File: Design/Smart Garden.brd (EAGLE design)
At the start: 92 x 87 mm, 96 parts, among them IC2 MP1584EN-LF-Z, IC3 CP2102, J1 USB-C, J2 POWER_JACK, T1 MMBT3904, T2 MMBT3904, T3 MMBT2222A, T4 MMBT2222A, T5 MMBT2222A, T6 MMBT2222A, U1 ESP-32S, U3 LM2596S, U4 DB107S

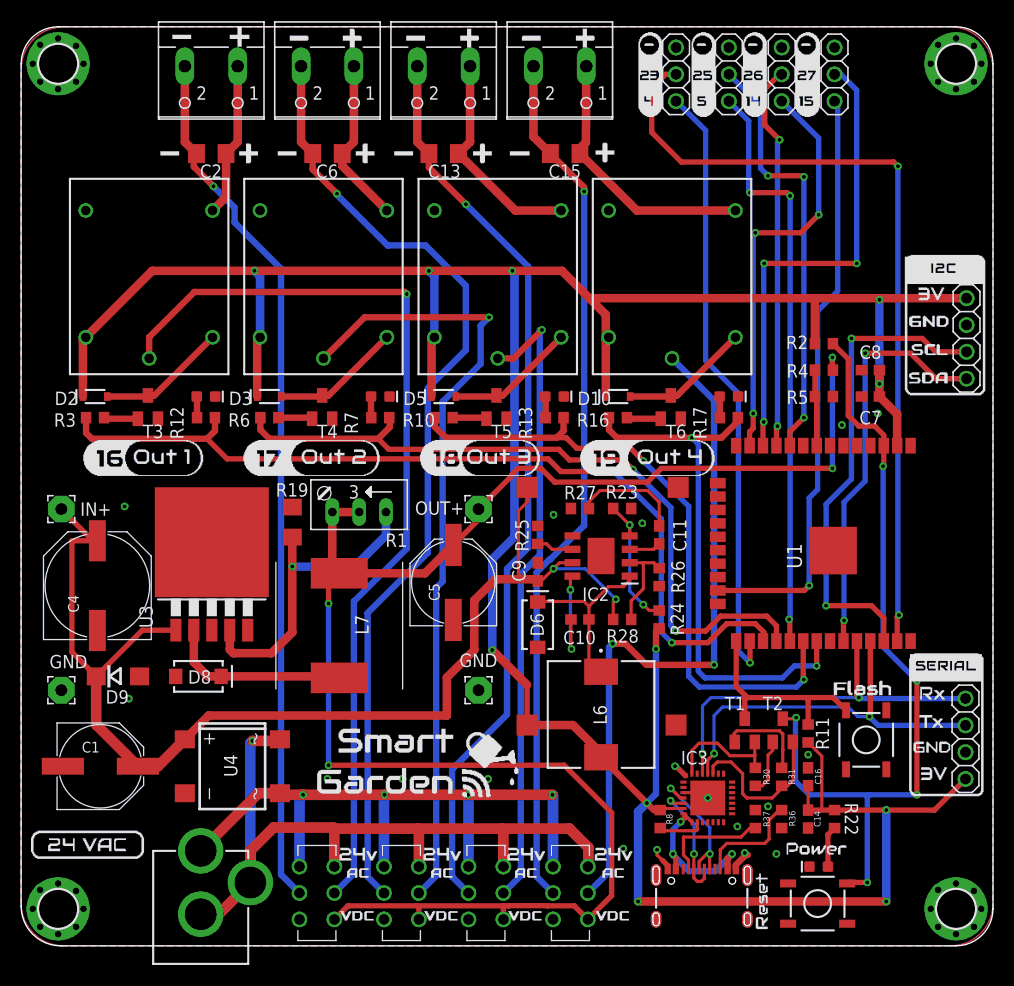
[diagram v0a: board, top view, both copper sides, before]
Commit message: Added V2R1 design files
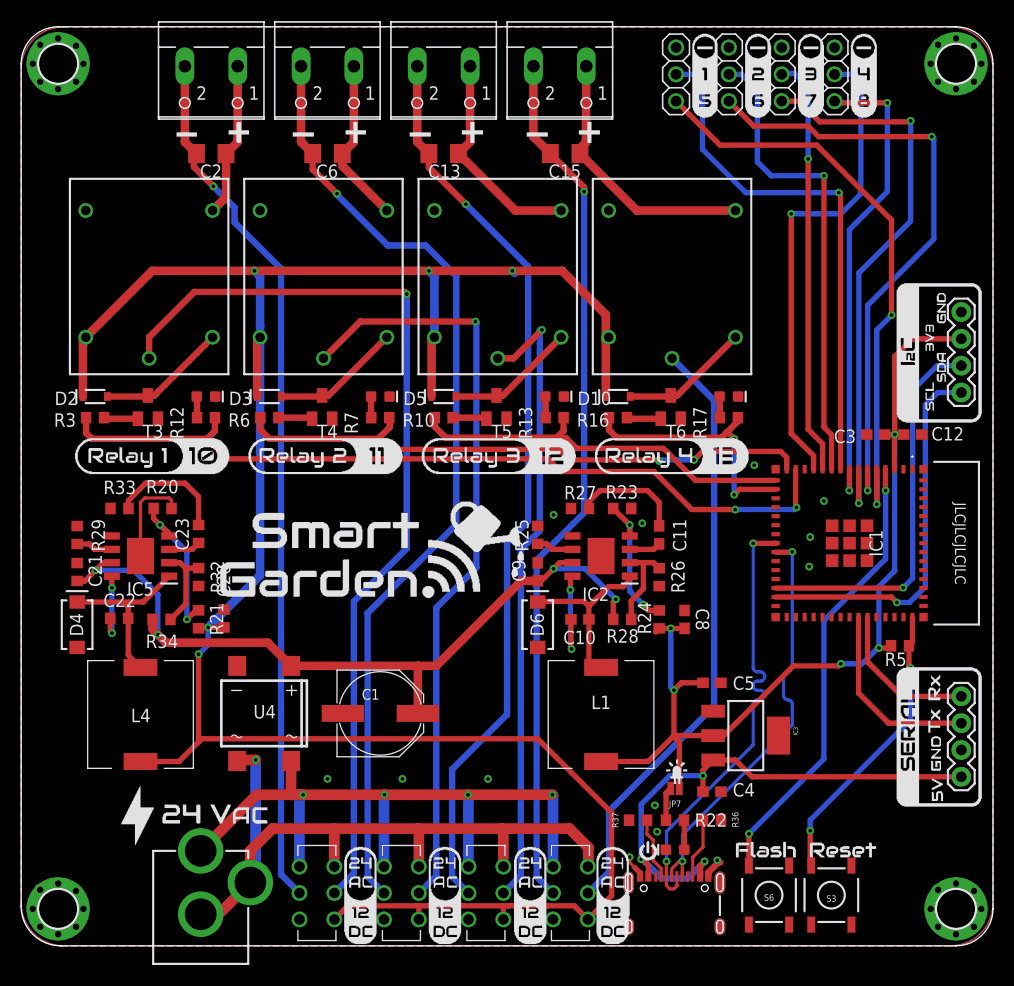
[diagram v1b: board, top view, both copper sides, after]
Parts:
- removed C14: 0.1uF, rcl:C0603
- removed C16: 4.7uF, rcl:C0603
- removed C7: 100nF, rcl:C0603
- removed D8: 3A/40V/500mV, SparkFun-DiscreteSemi:SMA-DIODE
- removed D9: US1M, diode:DO214AC
- removed JP1: Serial, SpaceDIY_connectors:1X04
- removed JP6: I2C, SpaceDIY_connectors:1X04
- removed L6: SLF10145T-100M2R5-H, SamacSys_Parts:SLF10145
- removed L7: 47µH, Wurth_Elektronik_Passive_rev15b:WE-PD_1260/1245/1280/1210
- removed PAD1, PAD2, PAD3, PAD4: (no value), wirepad:2,54/1,1
- removed R1: (no value), pot:RJ9W
- removed R11, R30, R31, R4, R8: 10k, rcl:R0603
- removed R19: 470R, rcl:R1206
- removed R2: 10K, rcl:R0603
- removed S1, S2: Reset, SpaceDIY_electromechanical:TACTILE_SWITCH_SMD_5.2MM
- removed T1, T2: MMBT3904, transistor-neu-to92:SOT23-BEC
- removed TP1, TP2, TP3, TP4: TPTP20SQ, testpad:TP20SQ
- removed U1: ESP-32S, esp32:ESP-32S
- removed U3: LM2596S, national-semiconductor:TO263-5
- added C12: 10uF, rcl:C0603
- added C20: 22uF, SpaceDIY_passive_components:0603
- added C21: 10uF, SpaceDIY_passive_components:0603
- added C22: 100nF, SpaceDIY_passive_components:0603
- added C23: 150pF, SpaceDIY_passive_components:0603
- added C3: 0.1uF, rcl:C0603
- added D4: 3A/40V/500mV, SparkFun-DiscreteSemi:SMA-DIODE
- added IC1: ESP32-S2-MINI-1-N4R2, SpaceDIY_modules:ESP32S2MINI1N4R2
- added IC5: MP1584EN-LF-Z, SamacSys_Parts:SOIC127P600X170-9N
- added J7, J9: (no value), SparkFun-Connectors:1X04
- added JP7: JUMPER-SMT_2_NC_PASTE_NO-SILK, SparkFun-Jumpers:SMT-JUMPER_2_NC_PASTE_NO-SILK
- added L1: CDRH104RNP-100NC, SpaceDIY_passive_components:CDRH104RNP
- added L4: CDRH104RNP-220NC, SpaceDIY_passive_components:CDRH104RNP
- added R20: 39k, SpaceDIY_passive_components:0603
- added R21: 560k, SpaceDIY_passive_components:0603
- added R29: 200k, SpaceDIY_passive_components:0603
- added R32: 24.9k, SpaceDIY_passive_components:0603
- added R33: 147k, SpaceDIY_passive_components:0603
- added R34: 100k, SpaceDIY_passive_components:0603
- added S3: Reset, SpaceDIY_electromechanical:TACTILE_SWITCH_SMD_5.2MM
- added S6: Flash, SpaceDIY_electromechanical:TACTILE_SWITCH_SMD_5.2MM
- C4: value 330µ/50V -> 10uF; device rcl:PANASONIC_G -> rcl:C0603
- C5: value 220µ/35V Low ESR -> 10uF; device rcl:PANASONIC_F -> rcl:C0603
- IC3: value CP2102 -> AMS1117-3.3; device silabs:MLP28 -> SparkFun-IC-Power:SOT223
- R10, R16, R3, R6: value 1.5k -> 1k
- R5: value 1.2k -> 10K
- RL1, RL3, RL5, RL7: value RELAYPTH -> SRD-12VDC-SL-C
- moved C4 61.4 mm to (65.4, 14.6), turned to 0 degrees
- moved C8 29.4 mm to (62.8, 30.9), turned to 90 degrees
- moved C1 27.0 mm to (34.0, 22.0)
- moved C5 26.3 mm to (65.4, 24.9), turned to 0 degrees
- moved R5 24.7 mm to (83.2, 28.4)
- moved R22 15.1 mm to (61.9, 11.9), turned to 180 degrees
- moved LED2 13.7 mm to (61.9, 9.10)
- moved R37 11.1 mm to (58.4, 11.9), turned to 0 degrees
- moved IC3 6.91 mm to (68.6, 19.9), turned to 270 degrees
- moved R36 6.60 mm to (65.4, 11.9), turned to 180 degrees
- moved U4 5.83 mm to (23.0, 22.0), turned to 180 degrees
- moved J1 2.69 mm to (61.8, 6.90)
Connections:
- removed net CLK: U1.20
- removed net CMD: U1.19
- removed net DTR: IC3.28, R30.1, T1.E
- removed net ESP_RST: R2.1, S2.3, T2.C, U1.3
- removed net IO12: U1.14
- removed net IO13: U1.16
- removed net IO14: JP3.3, U1.13
- removed net IO15: JP2.3, U1.23
- removed net IO16: R12.2, R3.2, U1.27
- removed net IO17: R6.2, R7.2, U1.28
- removed net IO18: R10.2, R13.2, U1.30
- removed net IO19: R16.2, R17.2, U1.31
- removed net IO2: U1.24
- removed net IO23: JP5.2, U1.37
- removed net IO25: JP4.2, U1.10
- removed net IO26: JP3.2, U1.11
- removed net IO27: JP2.2, U1.12
- removed net IO32: R4.1, R5.2, U1.8
- removed net IO33: U1.9
- removed net IO34: U1.6
- removed net IO35: U1.7
- removed net IO4: JP5.3, U1.26
- removed net IO5: JP4.3, U1.29
- removed net N$14: D8.C, L7.1, U3.2
- removed net N$18: R1.E, R19.2, U3.4
- removed net N$21: R30.2, T2.B
- removed net N$22: R31.2, T1.B
- removed net RTS: IC3.24, R31.1, T2.E
- removed net SD0: U1.21
- removed net SD1: U1.22
- removed net SD2: U1.17
- removed net SD3: U1.18
- removed net SVN: U1.5
- removed net SVP: U1.4
- removed net VCC: C5.+, L7.2, PAD3.1, R1.A, R1.S, R4.2, S4.1, S5.1, S7.1, S9.1
- removed net V_USB: IC3.7, IC3.8, J1.VBUS1, J1.VBUS2
- new net 12V: C20.1, D10.C, D2.C, D3.C, D5.C, L4.2, R21.2, RL1.COIL1, RL3.COIL1, RL5.COIL1, RL7.COIL1, S4.1, S5.1, S7.1, S9.1
- new net 5V: C4.1, IC3.3, J1.VBUS1, J1.VBUS2, J7.1
- new net IN_1: IC1.5, JP5.3
- new net IN_2: IC1.6, JP4.3
- new net IN_3: IC1.7, JP3.3
- new net IN_4: IC1.8, JP2.3
- new net N$25: C22.1, IC5.8
- new net N$26: C22.2, D4.C, IC5.1, L4.1
- new net N$41: IC5.4, R20.1, R21.1
- new net N$42: C23.2, R33.1
- new net N$43: C23.1, IC5.3
- new net N$44: IC5.6, R29.1
- new net N$45: IC5.2, R32.1, R34.2
- new net OUT_1: IC1.9, JP5.2
- new net OUT_2: IC1.10, JP4.2
- new net OUT_3: IC1.11, JP3.2
- new net OUT_4: IC1.12, JP2.2
- new net RELAY_1: IC1.14, R12.2, R3.2
- new net RELAY_2: IC1.15, R6.2, R7.2
- new net RELAY_3: IC1.16, R10.2, R13.2
- new net RELAY_4: IC1.17, R16.2, R17.2
- new net RST: IC1.45, R5.1, S3.3
- net 24V: now also C21.1, IC5.7, R34.1; no longer C4.+, D9.C, PAD1.1, TP1.TP, U3.1
- net 24V1: now also U4.AC2; no longer U4.AC1
- net 24V2: now also U4.AC1; no longer U4.AC2
- net 3.3V: now also C12.1, C3.1, C5.1, IC1.3, IC3.2, J9.2, JP7.1, L1.2, R5.2; no longer C14.1, C16.1, C7.1, D10.C, D2.C, D3.C, D5.C, IC3.6, JP1.4, JP6.4, L6.2, R11.1, R2.2, R22.2, R8.1, RL1.COIL1, RL3.COIL1, RL5.COIL1, RL7.COIL1, TP3.TP, U1.2
- net D+: now also IC1.24; no longer IC3.4
- net D-: now also IC1.23; no longer IC3.5
- net GND: now also C12.2, C20.2, C21.2, C3.2, C4.2, C5.2, D4.A, IC1.1, IC1.2, IC1.30, IC1.42, IC1.43, IC1.46, IC1.47, IC1.48, IC1.49, IC1.50, IC1.51, IC1.52, IC1.53, IC1.54, IC1.55, IC1.56, IC1.57, IC1.58, IC1.59, IC1.60, IC1.61, IC1.62, IC1.63, IC1.64, IC1.65, IC1.66, IC1.67, IC1.68, IC1.69, IC1.70, IC1.71, IC1.72, IC1.73, IC3.1, IC5.5, IC5.9, J7.2, J9.1, R20.2, R29.2, R32.2, R33.2, S3.1, S6.1; no longer C14.2, C16.2, C4.-, C5.-, C7.2, D8.A, D9.A, IC3.3, IC3.EXP, IC3.M, JP1.3, JP6.3, PAD2.1, PAD4.1, R19.1, R5.1, S1.1, S2.1, TP2.TP, TP4.TP, U1.1, U1.15, U1.38, U1.GND, U3.3, U3.5
- net IO0: now also IC1.4, S6.3; no longer R11.2, S1.3, T1.C, U1.25
- net N$35: now also L1.1; no longer L6.1
- net N$4: now also JP7.2, R22.2; no longer IC3.9, R8.2
- net RX: now also IC1.40, J7.4; no longer IC3.26, JP1.1, U1.34
- net SCL: now also IC1.29, J9.4; no longer JP6.2, U1.36
- net SDA: now also IC1.28, J9.3; no longer JP6.1, U1.33
- net TX: now also IC1.39, J7.3; no longer IC3.25, JP1.2, U1.35
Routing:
- net 12V: track 0.00 -> 222.5 mm, vias 0 -> 5
- net 3.3V: track 299.1 -> 93.6 mm, vias 11 -> 5
- net VCC: track 159.4 -> 0.00 mm, vias 4 -> 0
- net IO16: track 84.4 -> 0.00 mm, vias 2 -> 0
- net RELAY_1: track 0.00 -> 77.7 mm, vias 0 -> 2
- net IO23: track 76.7 -> 0.00 mm, vias 2 -> 0
- net ESP_RST: track 76.6 -> 0.00 mm, vias 5 -> 0
- net IO17: track 69.3 -> 0.00 mm, vias 2 -> 0
- net IO18: track 61.6 -> 0.00 mm, vias 2 -> 0
- net IN_2: track 0.00 -> 58.8 mm, vias 0 -> 2
- net IO4: track 58.1 -> 0.00 mm, vias 1 -> 0
- net RELAY_2: track 0.00 -> 56.4 mm, vias 0 -> 2
- net IO15: track 55.9 -> 0.00 mm, vias 1 -> 0
- net IN_1: track 0.00 -> 55.9 mm, vias 0 -> 2
- net IO5: track 55.6 -> 0.00 mm, vias 3 -> 0
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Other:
- board text removed: "GND"
- board text removed: "IN+"
- board text removed: "OUT+"
